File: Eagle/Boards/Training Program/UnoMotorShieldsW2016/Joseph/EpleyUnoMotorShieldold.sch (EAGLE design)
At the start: 7 parts, among them J1 ARDUINO_UNO_R3

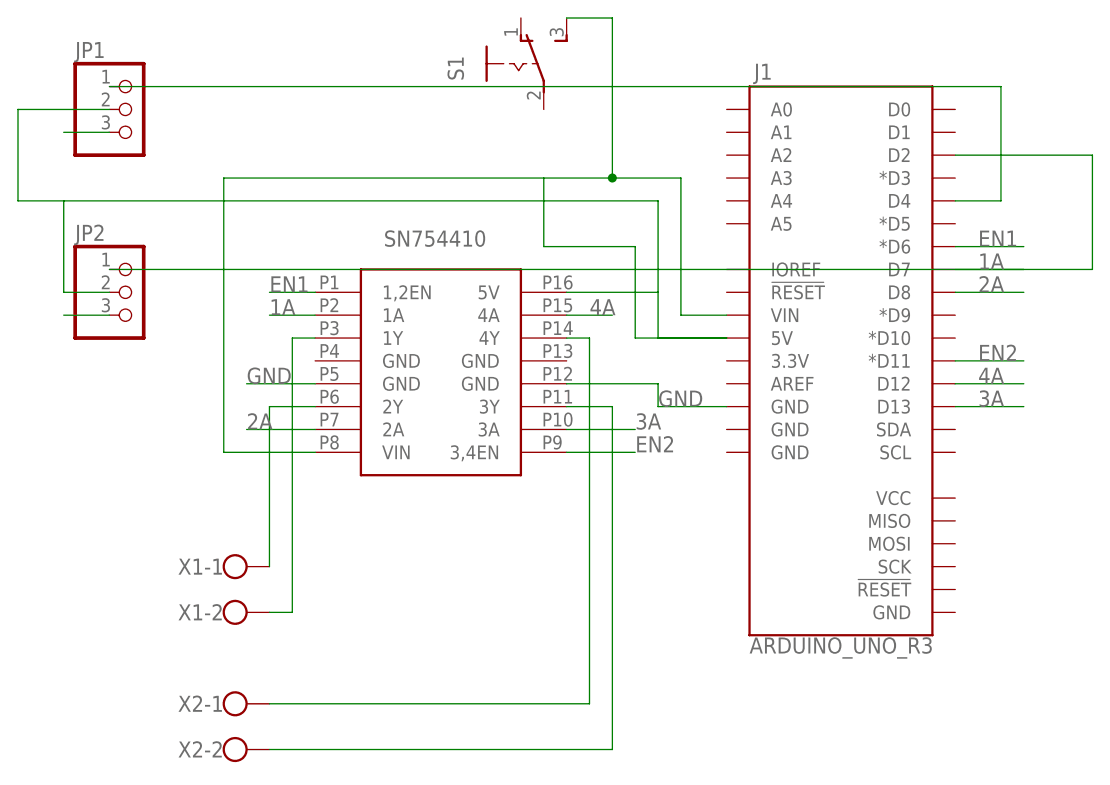
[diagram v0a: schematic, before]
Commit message: updated Joseph's board
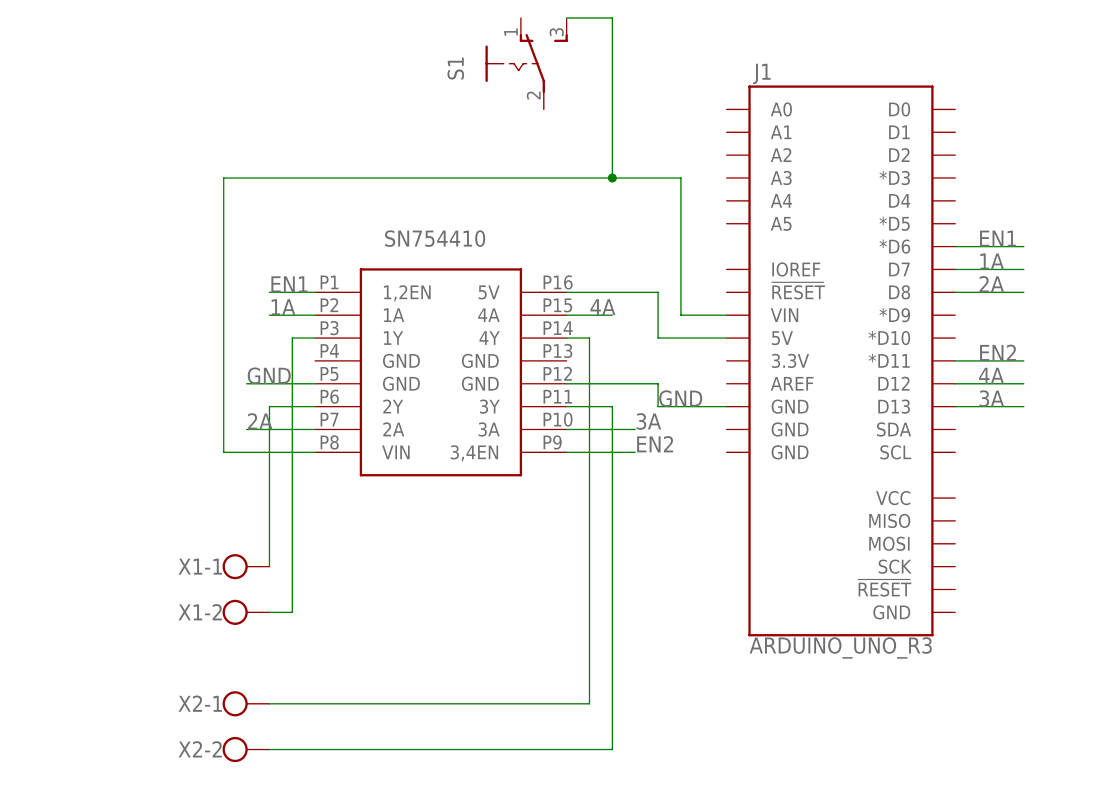
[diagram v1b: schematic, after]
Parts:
- removed JP1, JP2: (no value), ISCTRainingProgram:1X3HEADER
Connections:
- removed net N$11: J1.D4, JP1.1
- removed net N$12: J1.5V, JP1.2, JP2.2, U$1.5V
- net GND: no longer JP1.3, JP2.3
- net N$5: now also J1.5V, U$1.5V; no longer J1.D2, JP2.1
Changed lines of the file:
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@@
 <part name="X1" library="ISCTRainingProgram" deviceset="SCREWCONNECTOR" device=""/>
 <part name="X2" library="ISCTRainingProgram" deviceset="SCREWCONNECTOR" device=""/>
-<part name="JP1" library="ISCTRainingProgram" deviceset="1X3HEADER" device=""/>
-<part name="JP2" library="ISCTRainingProgram" deviceset="1X3HEADER" device=""/>
 </parts>
 <sheets>
@@
 <instance part="X2" gate="-1" x="2.54" y="27.94"/>
 <instance part="X2" gate="-2" x="2.54" y="22.86"/>
-<instance part="JP1" gate="A" x="-7.62" y="93.98"/>
-<instance part="JP2" gate="A" x="-7.62" y="73.66"/>
 </instances>
 <busses>
@@
 </segment>
 </net>
+<net name="N$5" class="0">
+<segment>
+<pinref part="J1" gate="G$1" pin="5V"/>
+<wire x1="58.42" y1="68.58" x2="50.8" y2="68.58" width="0.1524" layer="91"/>
+<wire x1="50.8" y1="68.58" x2="50.8" y2="73.66" width="0.1524" layer="91"/>
+<pinref part="U$1" gate="G$1" pin="5V"/>
+<wire x1="50.8" y1="73.66" x2="40.64" y2="73.66" width="0.1524" layer="91"/>
+</segment>
+</net>
 <net name="GND" class="0">
 <segment>
@@
 <wire x1="12.7" y1="63.5" x2="5.08" y2="63.5" width="0.1524" layer="91"/>
 <label x="5.08" y="63.5" size="1.778" layer="95"/>
-</segment>
-<segment>
-<pinref part="JP1" gate="A" pin="3"/>
-<wire x1="-10.16" y1="91.44" x2="-15.24" y2="91.44" width="0.1524" layer="91"/>
-</segment>
-<segment>
-<pinref part="JP2" gate="A" pin="3"/>
-<wire x1="-10.16" y1="71.12" x2="-15.24" y2="71.12" width="0.1524" layer="91"/>
 </segment>
 </net>
@@
 </segment>
 </net>
-<net name="N$10" class="0">
-<segment>
-<wire x1="38.1" y1="86.36" x2="38.1" y2="78.74" width="0.1524" layer="91"/>
-<wire x1="38.1" y1="78.74" x2="48.26" y2="78.74" width="0.1524" layer="91"/>
-<wire x1="48.26" y1="78.74" x2="48.26" y2="68.58" width="0.1524" layer="91"/>
-<wire x1="48.26" y1="68.58" x2="58.42" y2="68.58" width="0.1524" layer="91"/>
-</segment>
-</net>
-<net name="N$11" class="0">
-<segment>
-<pinref part="JP1" gate="A" pin="1"/>
-<wire x1="-10.16" y1="96.52" x2="88.9" y2="96.52" width="0.1524" layer="91"/>
-<wire x1="88.9" y1="96.52" x2="88.9" y2="83.82" width="0.1524" layer="91"/>
-<pinref part="J1" gate="G$1" pin="D4"/>
-<wire x1="88.9" y1="83.82" x2="83.82" y2="83.82" width="0.1524" layer="91"/>
-</segment>
-</net>
-<net name="N$12" class="0">
-<segment>
-<pinref part="JP1" gate="A" pin="2"/>
-<wire x1="-10.16" y1="93.98" x2="-20.32" y2="93.98" width="0.1524" layer="91"/>
-<wire x1="-20.32" y1="93.98" x2="-20.32" y2="83.82" width="0.1524" layer="91"/>
-<pinref part="J1" gate="G$1" pin="5V"/>
-<pinref part="U$1" gate="G$1" pin="5V"/>
-<wire x1="50.8" y1="73.66" x2="40.64" y2="73.66" width="0.1524" layer="91"/>
-<pinref part="JP2" gate="A" pin="2"/>
-<wire x1="-10.16" y1="73.66" x2="-15.24" y2="73.66" width="0.1524" layer="91"/>
-<wire x1="-15.24" y1="73.66" x2="-15.24" y2="83.82" width="0.1524" layer="91"/>
-<wire x1="-15.24" y1="83.82" x2="50.8" y2="83.82" width="0.1524" layer="91"/>
-<wire x1="50.8" y1="83.82" x2="50.8" y2="73.66" width="0.1524" layer="91"/>
-<wire x1="50.8" y1="73.66" x2="50.8" y2="68.58" width="0.1524" layer="91"/>
-<wire x1="50.8" y1="68.58" x2="58.42" y2="68.58" width="0.1524" layer="91"/>
-<wire x1="-20.32" y1="83.82" x2="-15.24" y2="83.82" width="0.1524" layer="91"/>
-</segment>
-</net>
-<net name="N$6" class="0">
-<segment>
-<wire x1="53.34" y1="68.58" x2="58.42" y2="68.58" width="0.1524" layer="91"/>
-</segment>
-</net>
-<net name="N$5" class="0">
-<segment>
-<pinref part="JP2" gate="A" pin="1"/>
-<wire x1="-10.16" y1="76.2" x2="99.06" y2="76.2" width="0.1524" layer="91"/>
-<wire x1="99.06" y1="76.2" x2="99.06" y2="88.9" width="0.1524" layer="91"/>
-<pinref part="J1" gate="G$1" pin="D2"/>
-<wire x1="99.06" y1="88.9" x2="83.82" y2="88.9" width="0.1524" layer="91"/>
-</segment>
-</net>
